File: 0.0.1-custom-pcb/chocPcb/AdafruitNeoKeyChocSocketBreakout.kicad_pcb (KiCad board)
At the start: 2 copper layers, 17.2 x 17.4 mm, 5 parts, among them J1 HC-FPC-0.5-6P-FH20, SW1 MX SOCKET

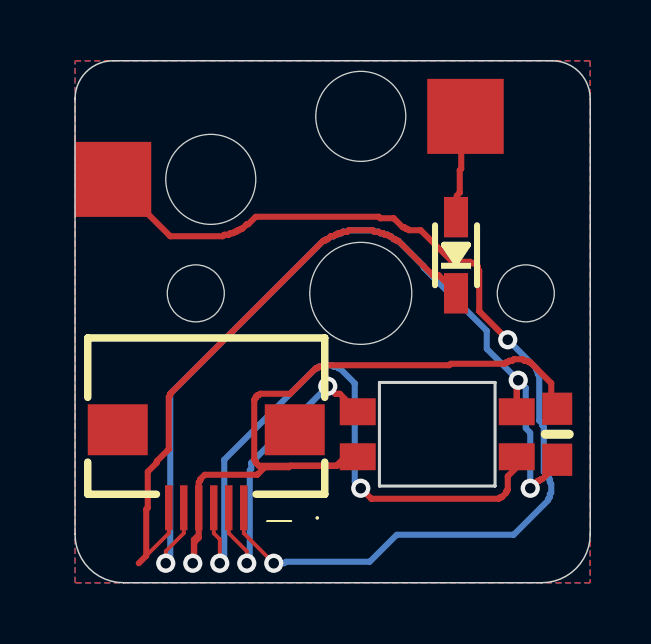
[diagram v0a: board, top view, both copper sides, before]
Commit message: choc rev1 looking good!
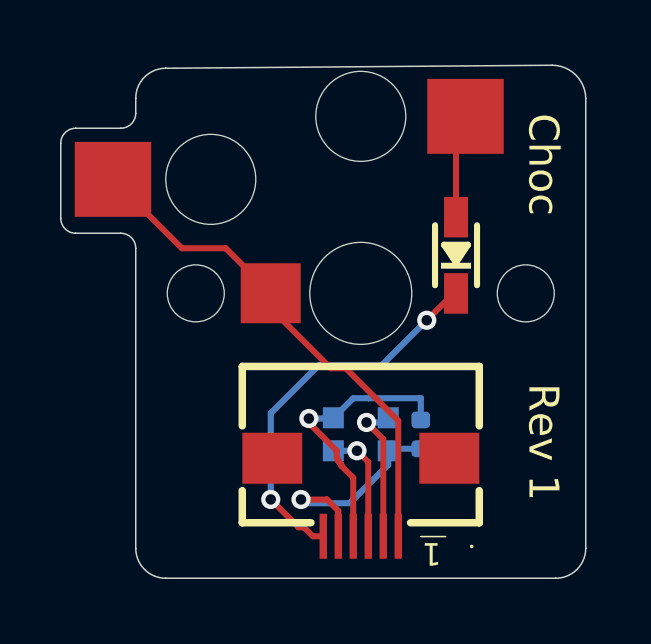
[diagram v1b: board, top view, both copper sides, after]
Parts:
- added TP1: TestPoint_Pad_2.0x2.0mm, ProjectParts:TestPoint_Pad_2.0x2.0mm, F.Cu at (145.5, 105.0)
- C1: value 1uF -> 100nF; footprint AdafruitNeoKeyChocSocketBreakout:0603-NO -> ProjectParts:C_0402_1005Metric; moved to B.Cu
- LED1: value WS2812B_SK6812E -> WS2812B-2020; footprint AdafruitNeoKeyChocSocketBreakout:NEO3535_REVERSE -> ProjectParts:LED_WS2812B-2020_PLCC4_2.0x2.0mm; moved to B.Cu
- moved J1 5.24 mm to (148.5, 111.8)
- moved C1 4.55 mm to (150.5, 109.7)
- moved LED1 2.55 mm to (148.5, 109.7)
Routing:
- net VDD: track 31.4 -> 7.52 mm, vias 3 -> 1
- net GND: track 27.8 -> 9.76 mm
- net NEO_OUT: track 21.4 -> 3.79 mm, vias 2 -> 1
- net SWITCHA: track 35.0 -> 17.8 mm, vias 2 -> 0
- net SWITCHC: track 21.1 -> 13.0 mm, vias 0 -> 2
- net NEO_IN: track 10.5 -> 5.12 mm, vias 2 -> 1
- removed copper zone on B.Cu, net GND
- removed copper zone on F.Cu, net GND
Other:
- board size 17.2 x 17.4 mm -> 17.5 x 17.1 mm
- board text added: "Choc"
- board text added: "Rev 1"
- board text removed: "Adafruit / FPC"
